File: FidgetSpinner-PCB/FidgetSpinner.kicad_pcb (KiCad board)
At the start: 2 copper layers, 81.9 x 90 mm, 41 parts, among them J1 DBG_CONN, SW1 SW_POWER, SW2 button, U1 STM32L010K8T6, U2 GP2S60

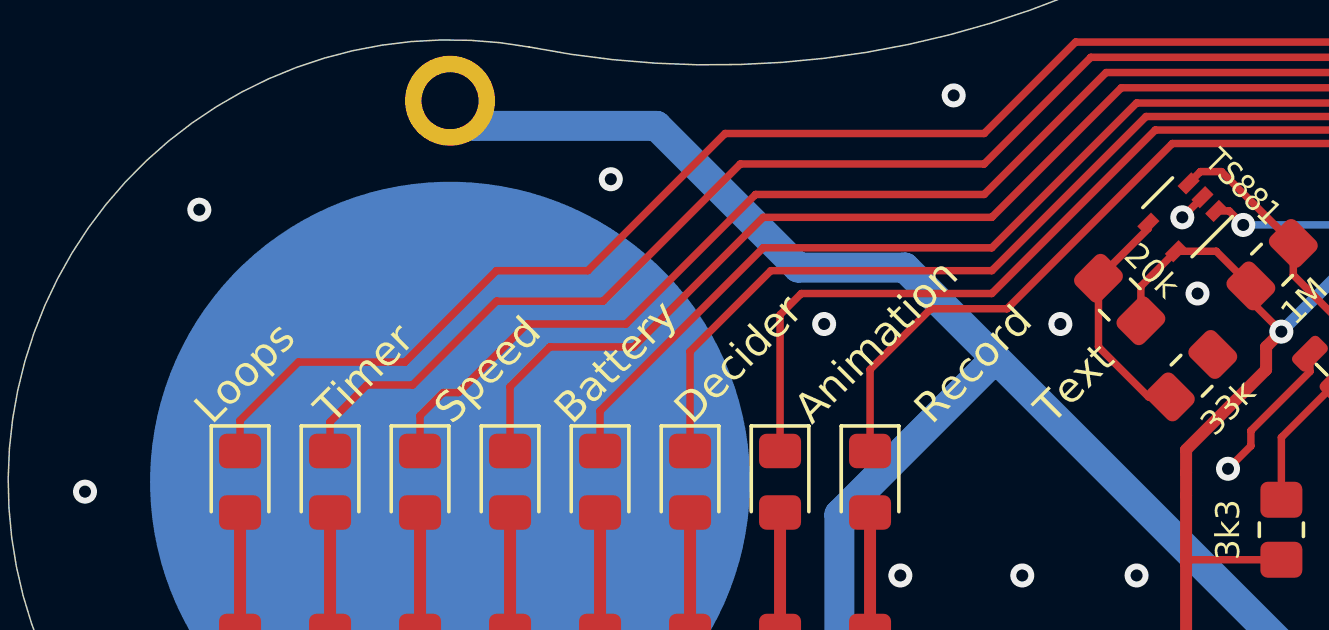
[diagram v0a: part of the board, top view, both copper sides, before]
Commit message: rearranged files
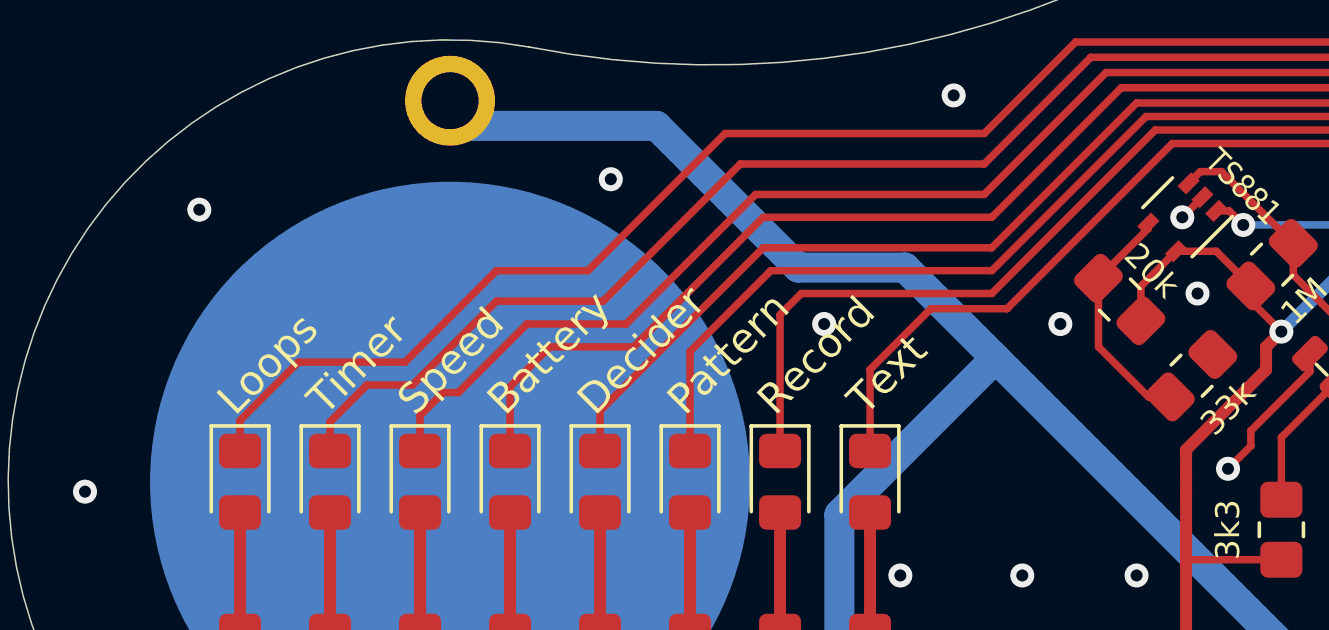
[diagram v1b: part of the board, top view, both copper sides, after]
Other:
- board text added: "Pattern"
- board text removed: "Animation"
